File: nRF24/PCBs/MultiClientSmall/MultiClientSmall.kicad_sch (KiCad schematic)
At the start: 17 parts, among them J1 Prog, M1 TP4056, SW1 SW_Push_Dual, U1 NRF24L01, U2 ATtiny84, U3 MCP1700x-330, U4 BH1750, U5 AM312, U6 BME280

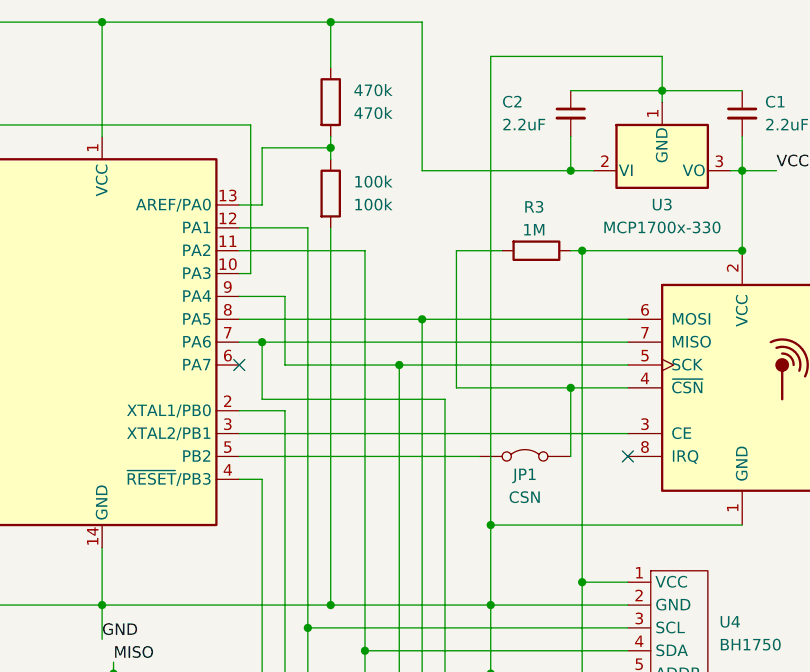
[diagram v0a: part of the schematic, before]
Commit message: nRF24 Multi-Client PCB V1.3
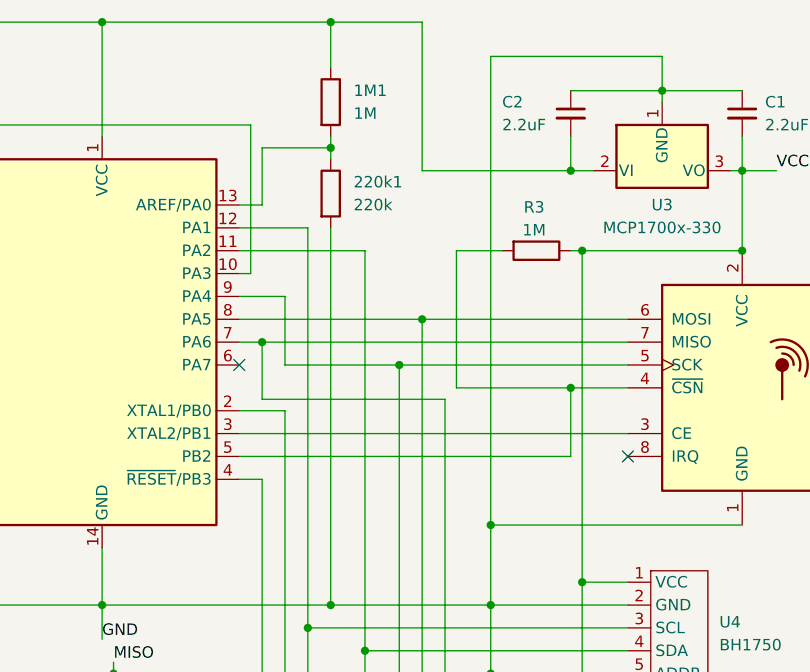
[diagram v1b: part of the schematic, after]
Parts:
- removed JP1: CSN, Connector_PinHeader_2.54mm:PinHeader_1x02_P2.54mm_Vertical, symbol Jumper:Jumper_2_Bridged
- 1M1: renamed from 470k; value 470k -> 1M
- 220k1: renamed from 100k; value 100k -> 220k
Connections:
- net at R3.2, U1.4 (~{CSN}): now also U2.5 (PB2)
